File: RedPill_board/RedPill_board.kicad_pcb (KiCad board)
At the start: 2 copper layers, 25.4 x 62.2 mm, 59 parts, among them J1 PROG, J2 USB_C_Receptacle_USB2.0, J3 Conn_01x22, J4 Conn_01x22, Q1 S9013, SW1 RESET, U1 FCM32F103CBT6, U2 ME6211C33M5G-N, U3 STM32F401RCT6, Y1 8MHz, Y2 8MHz

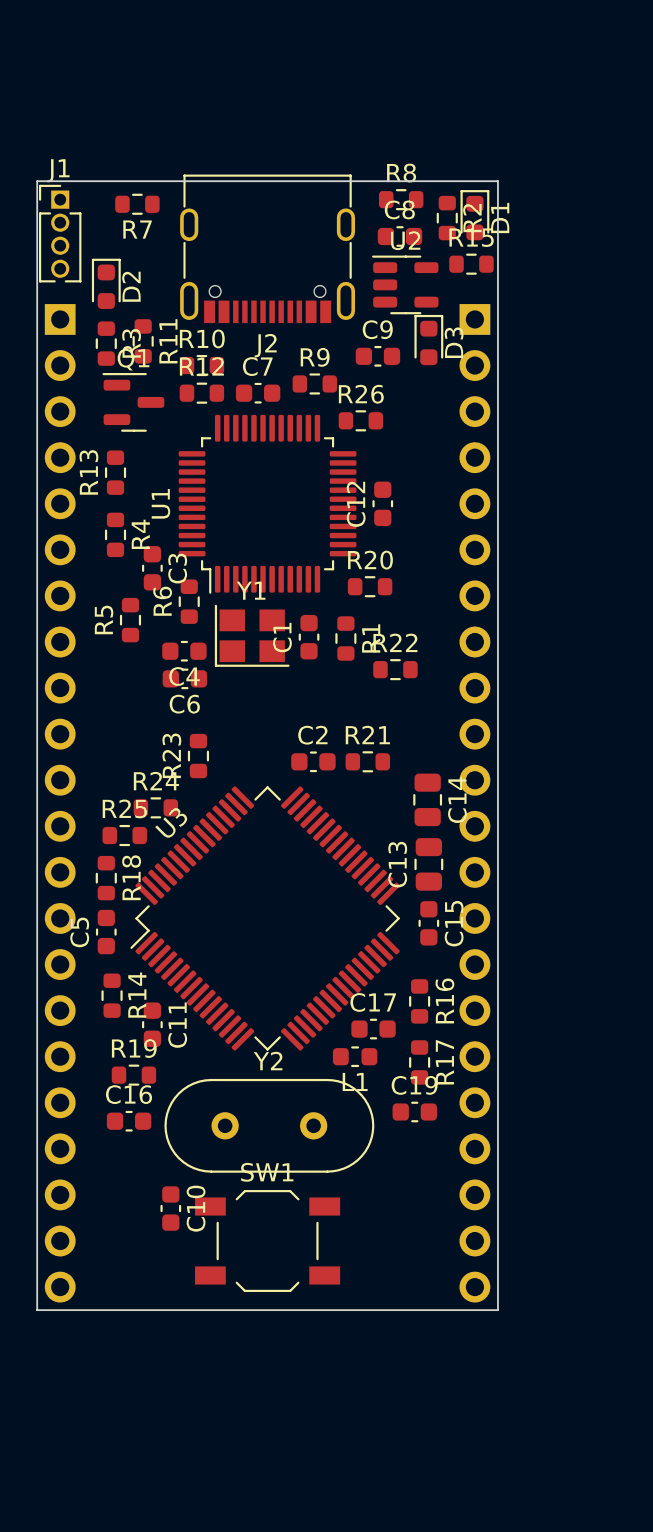
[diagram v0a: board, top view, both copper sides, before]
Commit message: Routing in progress.
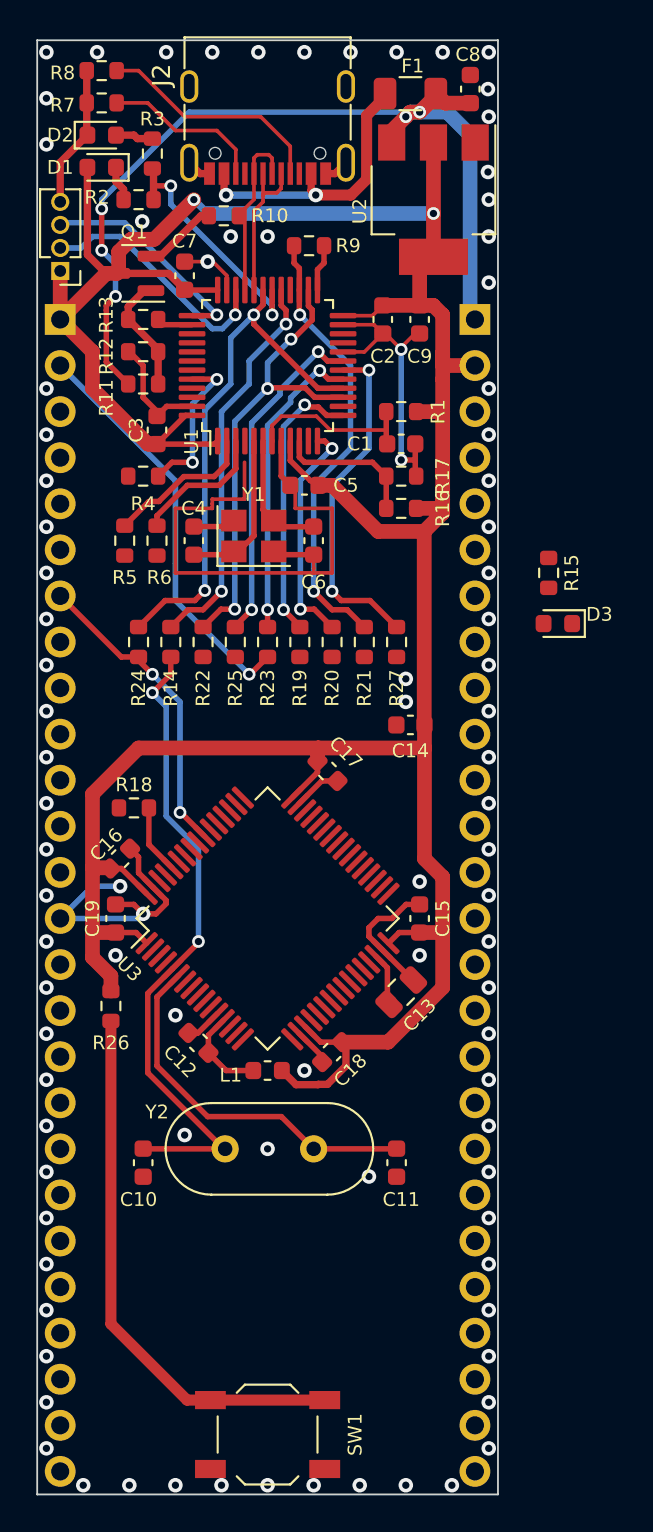
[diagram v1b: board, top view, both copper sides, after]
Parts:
- added C18: 100n, Capacitor_SMD:C_0603_1608Metric, F.Cu at (116.6, 109.0)
- added F1: 1A, Fuse:Fuse_1206_3216Metric, F.Cu at (120.9, 56.1)
- added R27: 22, Resistor_SMD:R_0603_1608Metric, F.Cu at (120.1, 86.4)
- C14: footprint Capacitor_SMD:C_0805_2012Metric -> Capacitor_SMD:C_0603_1608Metric
- J3, J4: value Conn_01x22 -> Conn_01x26; footprint Connector_PinHeader_2.54mm:PinHeader_1x22_P2.54mm_Vertical -> Connector_PinHeader_2.54mm:PinHeader_1x26_P2.54mm_Vertical
- R15, R2, R3: value 100 -> 220
- R26: value 100k -> 10k
- U1: value FCM32F103CBT6 -> STM32F103CBTx
- U2: value ME6211C33M5G-N -> AMS1117-3.3; footprint Package_TO_SOT_SMD:SOT-23-5 -> Package_TO_SOT_SMD:SOT-223-3_TabPin2
- moved R26 35.1 mm to (104.4, 106.4), turned to -90 degrees
- moved R17 32.3 mm to (120.4, 77.2), turned to 0 degrees
- moved C12 31.4 mm to (109.2, 108.5), turned to -45 degrees
- moved R16 27.2 mm to (120.4, 79.0), turned to 180 degrees
- moved C5 26.9 mm to (115.1, 77.7), turned to 180 degrees
- moved R19 25.6 mm to (114.8, 86.4), turned to -90 degrees
- moved C2 24.7 mm to (119.4, 68.6), turned to -90 degrees
- moved D1 20.8 mm to (103.9, 60.2), turned to 180 degrees
- moved R14 19.8 mm to (107.7, 86.4)
- moved C19 19.6 mm to (104.6, 101.6), turned to 90 degrees
- moved R8 18.0 mm to (103.9, 54.9), turned to 180 degrees
- moved R15 17.5 mm to (128.5, 82.5), turned to 90 degrees
- moved R2 17.0 mm to (105.9, 62.0), turned to 180 degrees
- moved D3 17.0 mm to (129.0, 85.3), turned to 180 degrees
- moved C11 15.5 mm to (120.1, 115.1)
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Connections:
- C12 pad 1: /T_NRST -> GND
- C12 pad 2: GND -> Net-(U3-VREF+)
- J2 pad A4: +5V -> Net-(F1-Pad1)
- J2 pad A9: +5V -> Net-(F1-Pad1)
- J2 pad B4: +5V -> Net-(F1-Pad1)
- J2 pad B9: +5V -> Net-(F1-Pad1)
- J3 pad 1: unconnected-(J3-Pin_1-Pad1) -> +3V3
- J3 pad 10: unconnected-(J3-Pin_10-Pad10) -> /PB6
- J3 pad 11: unconnected-(J3-Pin_11-Pad11) -> /PB7
- J3 pad 12: unconnected-(J3-Pin_12-Pad12) -> /PB8
- J3 pad 13: unconnected-(J3-Pin_13-Pad13) -> /PB9
- J3 pad 14: unconnected-(J3-Pin_14-Pad14) -> GND
- J3 pad 15: unconnected-(J3-Pin_15-Pad15) -> /PC13
- J3 pad 16: unconnected-(J3-Pin_16-Pad16) -> /PC14
- J3 pad 17: unconnected-(J3-Pin_17-Pad17) -> /PC15
- J3 pad 18: unconnected-(J3-Pin_18-Pad18) -> /PC0
- J3 pad 19: unconnected-(J3-Pin_19-Pad19) -> /PC1
- J3 pad 2: unconnected-(J3-Pin_2-Pad2) -> /PA15
- J3 pad 20: unconnected-(J3-Pin_20-Pad20) -> /PC2
- J3 pad 21: unconnected-(J3-Pin_21-Pad21) -> /PC3
- J3 pad 22: unconnected-(J3-Pin_22-Pad22) -> /PA0
- J3 pad 3: unconnected-(J3-Pin_3-Pad3) -> /PC10
- J3 pad 4: unconnected-(J3-Pin_4-Pad4) -> /PC11
- J3 pad 5: unconnected-(J3-Pin_5-Pad5) -> /PC12
- J3 pad 6: unconnected-(J3-Pin_6-Pad6) -> /PD2
- J3 pad 7: unconnected-(J3-Pin_7-Pad7) -> /PB3
- J3 pad 8: unconnected-(J3-Pin_8-Pad8) -> /PB4
- J3 pad 9: unconnected-(J3-Pin_9-Pad9) -> /PB5
- J4 pad 1: unconnected-(J4-Pin_1-Pad1) -> +5V
- J4 pad 10: unconnected-(J4-Pin_10-Pad10) -> /PC7
- J4 pad 11: unconnected-(J4-Pin_11-Pad11) -> /PC6
- J4 pad 12: unconnected-(J4-Pin_12-Pad12) -> /PB15
- J4 pad 13: unconnected-(J4-Pin_13-Pad13) -> /PB14
- J4 pad 14: unconnected-(J4-Pin_14-Pad14) -> /PB13
- J4 pad 15: unconnected-(J4-Pin_15-Pad15) -> /PB12
- J4 pad 16: unconnected-(J4-Pin_16-Pad16) -> /PB10
- J4 pad 17: unconnected-(J4-Pin_17-Pad17) -> /PB2
- J4 pad 18: unconnected-(J4-Pin_18-Pad18) -> /PB1
- J4 pad 19: unconnected-(J4-Pin_19-Pad19) -> /PB0
- J4 pad 2: unconnected-(J4-Pin_2-Pad2) -> +3V3
- J4 pad 20: unconnected-(J4-Pin_20-Pad20) -> /PC5
- J4 pad 21: unconnected-(J4-Pin_21-Pad21) -> /PC4
- J4 pad 22: unconnected-(J4-Pin_22-Pad22) -> /PA7
- J4 pad 3: unconnected-(J4-Pin_3-Pad3) -> /PA12
- J4 pad 4: unconnected-(J4-Pin_4-Pad4) -> /PA11
- J4 pad 5: unconnected-(J4-Pin_5-Pad5) -> /PA10
- J4 pad 6: unconnected-(J4-Pin_6-Pad6) -> /PA9
- J4 pad 7: unconnected-(J4-Pin_7-Pad7) -> /PA8
- J4 pad 8: unconnected-(J4-Pin_8-Pad8) -> /PC9
- J4 pad 9: unconnected-(J4-Pin_9-Pad9) -> /PC8
- R19 pad 2: /USART_TX -> /PA2
- R20 pad 2: /USART_RX -> /PA3
- R23 pad 1: Net-(U3-PA15) -> /PA15
- R24 pad 2: Net-(U3-PB3) -> /PB3
- R25 pad 2: Net-(U3-PB4) -> /PB4
- R26 pad 2: /T_NRST -> Net-(U3-NRST)
- SW1 pad 1: /T_NRST -> Net-(U3-NRST)
- U1 pad 1: unconnected-(U1-NC-Pad1) -> +3V3
- U2 pad 1: +5V -> GND
- U2 pad 2: GND -> +3V3
- U3 pad 10: unconnected-(U3-PC2-Pad10) -> /PC2
- U3 pad 11: unconnected-(U3-PC3-Pad11) -> /PC3
- U3 pad 14: unconnected-(U3-PA0-Pad14) -> /PA0
- U3 pad 15: unconnected-(U3-PA1-Pad15) -> /PA1
- U3 pad 16: /USART_TX -> /PA2
- U3 pad 17: /USART_RX -> /PA3
- U3 pad 2: unconnected-(U3-PC13-Pad2) -> /PC13
- U3 pad 20: unconnected-(U3-PA4-Pad20) -> /PA4
- U3 pad 21: unconnected-(U3-PA5-Pad21) -> /PA5
- U3 pad 22: unconnected-(U3-PA6-Pad22) -> /PA6
- U3 pad 23: unconnected-(U3-PA7-Pad23) -> /PA7
- U3 pad 24: unconnected-(U3-PC4-Pad24) -> /PC4
- U3 pad 25: unconnected-(U3-PC5-Pad25) -> /PC5
- U3 pad 26: unconnected-(U3-PB0-Pad26) -> /PB0
- U3 pad 27: unconnected-(U3-PB1-Pad27) -> /PB1
- U3 pad 28: unconnected-(U3-PB2-Pad28) -> /PB2
- U3 pad 29: unconnected-(U3-PB10-Pad29) -> /PB10
- U3 pad 3: unconnected-(U3-PC14-Pad3) -> /PC14
- U3 pad 33: unconnected-(U3-PB12-Pad33) -> /PB12
- U3 pad 34: unconnected-(U3-PB13-Pad34) -> /PB13
- U3 pad 35: unconnected-(U3-PB14-Pad35) -> /PB14
- U3 pad 36: unconnected-(U3-PB15-Pad36) -> /PB15
- U3 pad 37: unconnected-(U3-PC6-Pad37) -> /PC6
- U3 pad 38: unconnected-(U3-PC7-Pad38) -> /PC7
- U3 pad 39: unconnected-(U3-PC8-Pad39) -> /PC8
- U3 pad 4: unconnected-(U3-PC15-Pad4) -> /PC15
- U3 pad 40: unconnected-(U3-PC9-Pad40) -> /PC9
- U3 pad 41: unconnected-(U3-PA8-Pad41) -> /PA8
- U3 pad 42: unconnected-(U3-PA9-Pad42) -> /PA9
- U3 pad 43: unconnected-(U3-PA10-Pad43) -> /PA10
- U3 pad 44: unconnected-(U3-PA11-Pad44) -> /PA11
- U3 pad 45: unconnected-(U3-PA12-Pad45) -> /PA12
- U3 pad 50: Net-(U3-PA15) -> /PA15
- U3 pad 51: unconnected-(U3-PC10-Pad51) -> /PC10
- U3 pad 52: unconnected-(U3-PC11-Pad52) -> /PC11
- U3 pad 53: unconnected-(U3-PC12-Pad53) -> /PC12
- U3 pad 54: unconnected-(U3-PD2-Pad54) -> /PD2
- U3 pad 55: Net-(U3-PB3) -> /PB3
- U3 pad 56: Net-(U3-PB4) -> /PB4
- U3 pad 57: unconnected-(U3-PB5-Pad57) -> /PB5
- U3 pad 58: unconnected-(U3-PB6-Pad58) -> /PB6
- U3 pad 59: unconnected-(U3-PB7-Pad59) -> /PB7
- U3 pad 61: unconnected-(U3-PB8-Pad61) -> /PB8
- U3 pad 62: unconnected-(U3-PB9-Pad62) -> /PB9
- U3 pad 7: /T_NRST -> Net-(U3-NRST)
- U3 pad 8: unconnected-(U3-PC0-Pad8) -> /PC0
- U3 pad 9: unconnected-(U3-PC1-Pad9) -> /PC1
- Y1 pad 2: /PGM_OSC_OUT -> GND
- Y1 pad 3: (no net) -> /PGM_OSC_OUT
- Y1 pad 4: (no net) -> GND
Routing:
- net +3V3: track 0.00 -> 183.1 mm, vias 0 -> 2
- net GND: track 0.00 -> 100.3 mm, vias 0 -> 93
- net +5V: track 0.00 -> 50.6 mm, vias 0 -> 5
- net /MCO: track 0.00 -> 36.1 mm, vias 0 -> 2
- net Net-(U3-NRST): track 0.00 -> 30.2 mm
- net /T_JTDO_SWO: track 0.00 -> 29.3 mm, vias 0 -> 2
- net /T_JTCK_SWCLK: track 0.00 -> 26.1 mm, vias 0 -> 3
- net /T_JTMS_SWDIO: track 0.00 -> 24.8 mm, vias 0 -> 2
- net /PA15: track 0.00 -> 22.7 mm, vias 0 -> 1
- net Net-(U1-PA8): track 0.00 -> 21.8 mm, vias 0 -> 2
- net Net-(U3-PH1): track 0.00 -> 20.6 mm
- net /T_NRST: track 0.00 -> 18.8 mm, vias 0 -> 2
- net /T_JRST: track 0.00 -> 18.7 mm, vias 0 -> 2
- net /PB3: track 0.00 -> 17.1 mm, vias 0 -> 2
- net /T_JTDI: track 0.00 -> 16.9 mm, vias 0 -> 2
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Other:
- board size 25.4 x 62.2 mm -> 25.4 x 80.2 mm
